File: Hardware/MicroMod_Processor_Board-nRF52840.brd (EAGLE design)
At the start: 22 x 22 mm, 30 parts, among them J2 MICROMOD-2222, U1 W25QXX128MBIT-6X5, U2 MDBT50Q, Y1 32.768kHz

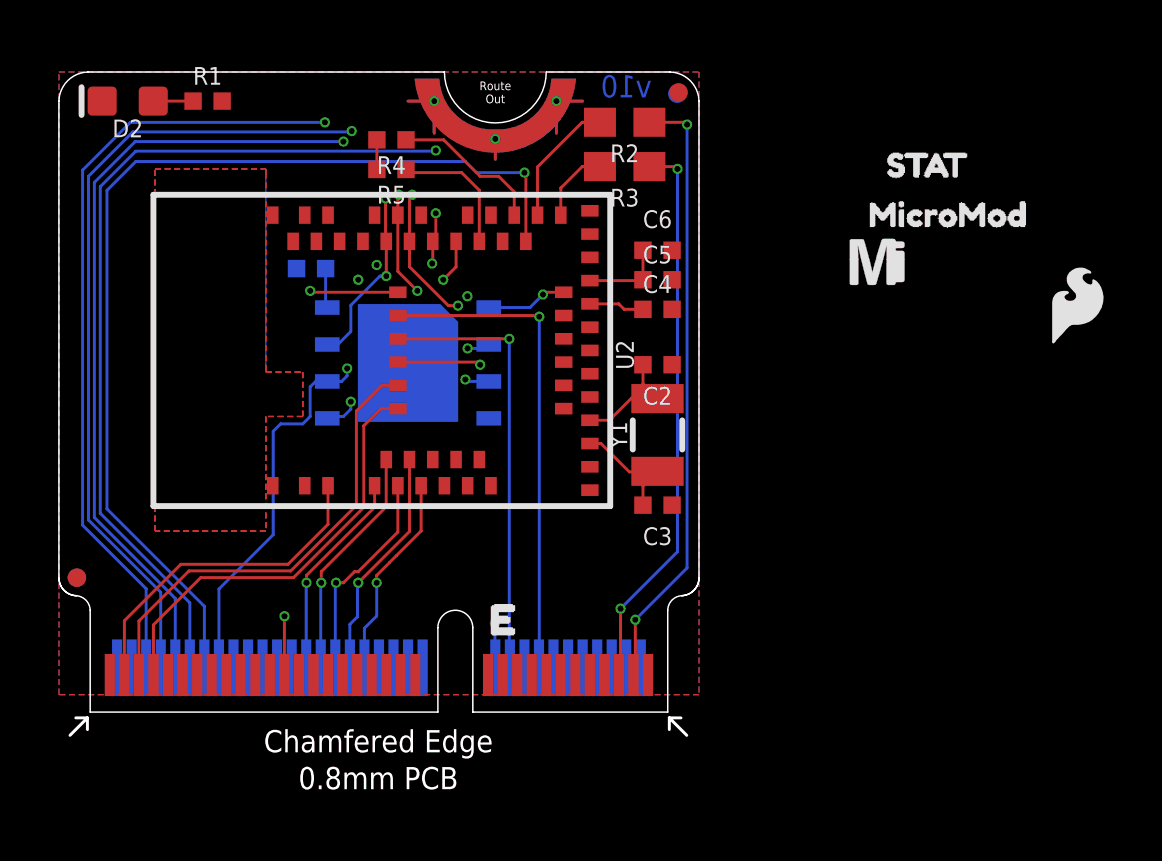
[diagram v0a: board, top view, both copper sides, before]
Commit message: Routing
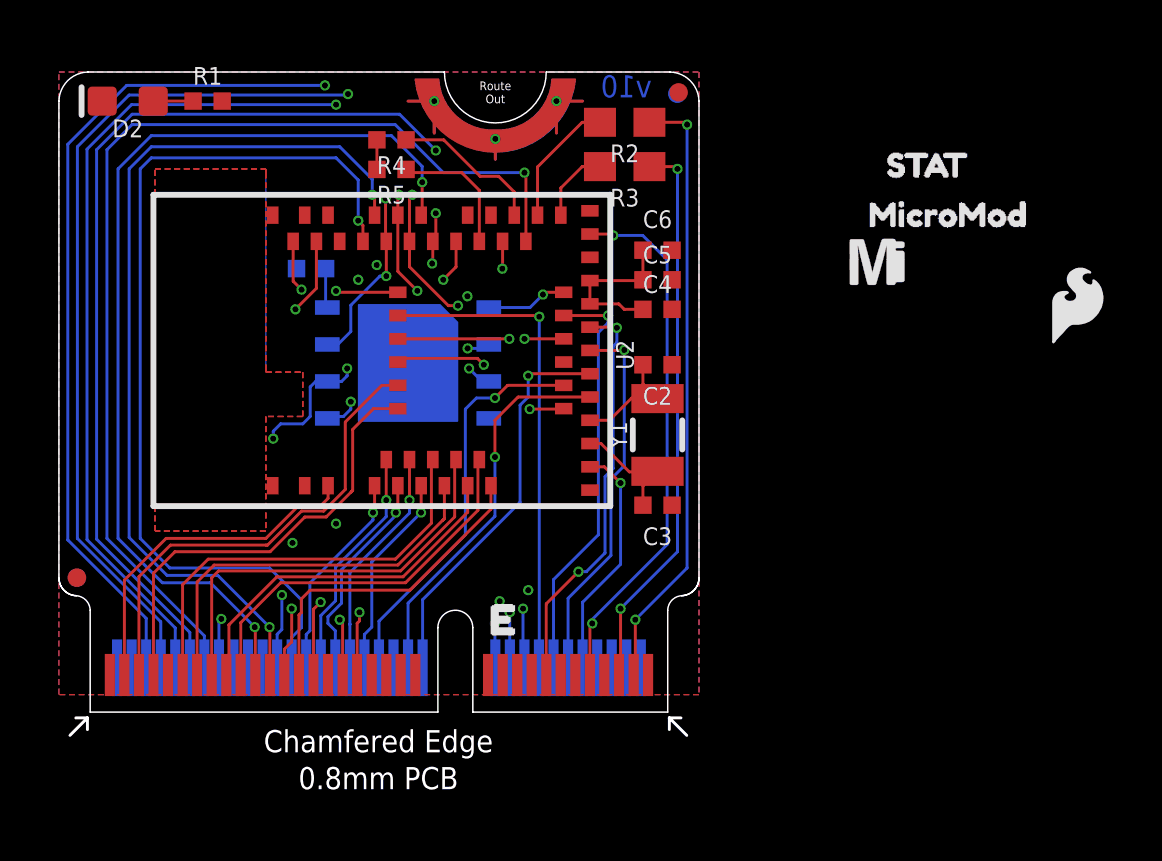
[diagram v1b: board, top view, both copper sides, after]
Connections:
- net ADC_D+: now also U2.10; no longer U2.13
- net ADC_D-: now also U2.9; no longer U2.11
- net BATT_VIN/3: now also U2.14; no longer U2.10
- net CTS1: now also U2.26; no longer U2.22
- net PWM0: now also U2.22; no longer U2.26
- net SPI_MISO1: now also U2.11; no longer U2.12
- net SPI_MOSI1: now also U2.12; no longer U2.9
- net SPI_SCK1: now also U2.13; no longer U2.14
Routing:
- net SPI_!CS!1: track 0.00 -> 33.4 mm, vias 0 -> 2
- net PDM_CLK: track 0.00 -> 31.7 mm, vias 0 -> 1
- net SCL1: track 0.00 -> 30.8 mm, vias 0 -> 2
- net PWM1: track 0.00 -> 21.5 mm, vias 0 -> 3
- net PDM_DATA: track 0.00 -> 18.5 mm, vias 0 -> 3
- net USB_VIN: track 0.00 -> 18.4 mm, vias 0 -> 2
- net NFC2: track 0.00 -> 15.9 mm, vias 0 -> 2
- net NFC1: track 0.00 -> 15.9 mm, vias 0 -> 2
- net ADC_D-: track 0.00 -> 14.7 mm
- net SPI_MISO1: track 0.00 -> 14.5 mm
- net SCL: track 0.00 -> 14.4 mm, vias 0 -> 1
- net CTS1: track 0.00 -> 14.0 mm, vias 0 -> 2
- net ADC1: track 0.00 -> 13.8 mm, vias 0 -> 1
- net ADC_D+: track 0.00 -> 13.7 mm
- net PWM0: track 0.00 -> 13.7 mm, vias 0 -> 1
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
